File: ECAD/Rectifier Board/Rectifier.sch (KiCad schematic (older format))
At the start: 21 parts

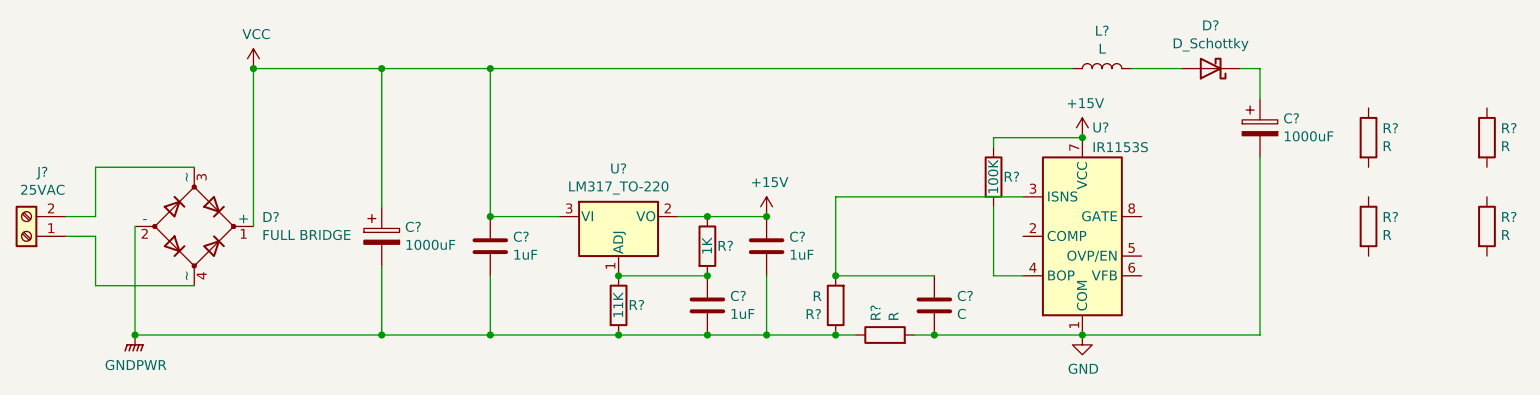
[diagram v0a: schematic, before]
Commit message: Cin
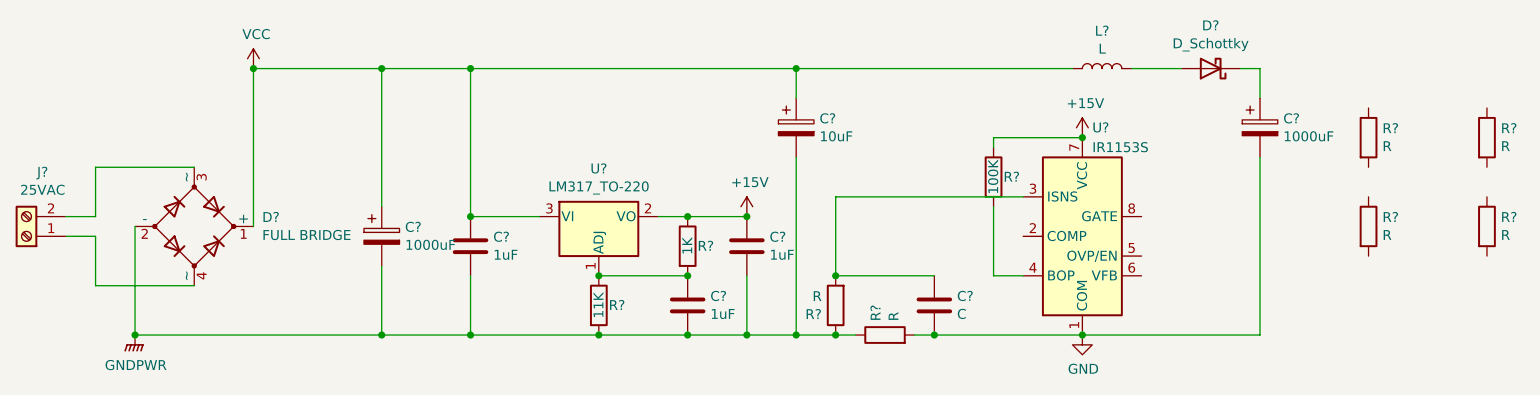
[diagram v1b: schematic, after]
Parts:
- added C?: 10uF, symbol Device:CP
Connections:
- net GNDPWR: now also C?.2
- net VCC: now also C?.1
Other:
- moved on the sheet: C?, R?, U?
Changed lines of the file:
@@
 L Regulator_Linear:LM317_TO-220 U?
 U 1 1 6205D4E8
-P 5150 2900
-F 0 "U?" H 5150 3142 50  0000 C CNN
-F 1 "LM317_TO-220" H 5150 3051 50  0000 C CNN
-F 2 "Package_TO_SOT_THT:TO-220-3_Vertical" H 5150 3150 50  0001 C CIN
-F 3 "http://www.ti.com/lit/ds/symlink/lm317.pdf" H 5150 2900 50  0001 C CNN
-	1    5150 2900
+P 5050 2900
+F 0 "U?" H 5050 3142 50  0000 C CNN
+F 1 "LM317_TO-220" H 5050 3051 50  0000 C CNN
+F 2 "Package_TO_SOT_THT:TO-220-3_Vertical" H 5050 3150 50  0001 C CIN
+F 3 "http://www.ti.com/lit/ds/symlink/lm317.pdf" H 5050 2900 50  0001 C CNN
+	1    5050 2900
 	1    0    0    -1
 $EndComp
@@
 L Device:R R?
 U 1 1 6205E083
-P 5150 3350
-F 0 "R?" H 5200 3350 50  0000 L CNN
-F 1 "11K" V 5150 3350 50  0000 C CNN
-F 2 "" V 5080 3350 50  0001 C CNN
-F 3 "~" H 5150 3350 50  0001 C CNN
-	1    5150 3350
+P 5050 3350
+F 0 "R?" H 5100 3350 50  0000 L CNN
+F 1 "11K" V 5050 3350 50  0000 C CNN
+F 2 "" V 4980 3350 50  0001 C CNN
+F 3 "~" H 5050 3350 50  0001 C CNN
+	1    5050 3350
 	1    0    0    -1
 $EndComp
@@
 L Device:R R?
 U 1 1 6205F378
-P 5600 3050
-F 0 "R?" H 5650 3050 50  0000 L CNN
-F 1 "1K" V 5600 3050 50  0000 C CNN
-F 2 "" V 5530 3050 50  0001 C CNN
-F 3 "~" H 5600 3050 50  0001 C CNN
-	1    5600 3050
-	1    0    0    -1
-$EndComp
-Wire Wire Line
-	5150 3200 5600 3200
-Connection ~ 5150 3200
-Wire Wire Line
-	5600 2900 5450 2900
+P 5500 3050
+F 0 "R?" H 5550 3050 50  0000 L CNN
+F 1 "1K" V 5500 3050 50  0000 C CNN
+F 2 "" V 5430 3050 50  0001 C CNN
+F 3 "~" H 5500 3050 50  0001 C CNN
+	1    5500 3050
+	1    0    0    -1
+$EndComp
+Wire Wire Line
+	5050 3200 5500 3200
+Connection ~ 5050 3200
+Wire Wire Line
+	5500 2900 5350 2900
 $Comp
 L Device:C C?
 U 1 1 6205FE8A
-P 5900 3050
-F 0 "C?" H 6015 3096 50  0000 L CNN
-F 1 "1uF" H 6015 3005 50  0000 L CNN
-F 2 "" H 5938 2900 50  0001 C CNN
-F 3 "~" H 5900 3050 50  0001 C CNN
-	1    5900 3050
+P 5800 3050
+F 0 "C?" H 5915 3096 50  0000 L CNN
+F 1 "1uF" H 5915 3005 50  0000 L CNN
+F 2 "" H 5838 2900 50  0001 C CNN
+F 3 "~" H 5800 3050 50  0001 C CNN
+	1    5800 3050
 	1    0    0    -1
 $EndComp
@@
 L Device:C C?
 U 1 1 620613FC
-P 5600 3350
-F 0 "C?" H 5715 3396 50  0000 L CNN
-F 1 "1uF" H 5715 3305 50  0000 L CNN
-F 2 "" H 5638 3200 50  0001 C CNN
-F 3 "~" H 5600 3350 50  0001 C CNN
-	1    5600 3350
-	1    0    0    -1
-$EndComp
-Connection ~ 5600 3200
-Wire Wire Line
-	5150 3500 5600 3500
-Wire Wire Line
-	5600 3500 5900 3500
-Wire Wire Line
-	5900 3500 5900 3200
-Connection ~ 5600 3500
-Wire Wire Line
-	5900 2900 5600 2900
-Connection ~ 5600 2900
+P 5500 3350
+F 0 "C?" H 5615 3396 50  0000 L CNN
+F 1 "1uF" H 5615 3305 50  0000 L CNN
+F 2 "" H 5538 3200 50  0001 C CNN
+F 3 "~" H 5500 3350 50  0001 C CNN
+	1    5500 3350
+	1    0    0    -1
+$EndComp
+Connection ~ 5500 3200
+Wire Wire Line
+	5800 3500 5800 3200
+Wire Wire Line
+	5800 2900 5500 2900
+Connection ~ 5500 2900
 $Comp
 L Device:C C?
 U 1 1 620625CD
-P 4500 3050
-F 0 "C?" H 4615 3096 50  0000 L CNN
-F 1 "1uF" H 4615 3005 50  0000 L CNN
-F 2 "" H 4538 2900 50  0001 C CNN
-F 3 "~" H 4500 3050 50  0001 C CNN
-	1    4500 3050
-	1    0    0    -1
-$EndComp
-Wire Wire Line
-	4500 3500 4500 3200
-Wire Wire Line
-	4850 2900 4500 2900
-Wire Wire Line
-	4500 3500 5150 3500
-Connection ~ 5150 3500
+P 4400 3050
+F 0 "C?" H 4515 3096 50  0000 L CNN
+F 1 "1uF" H 4515 3005 50  0000 L CNN
+F 2 "" H 4438 2900 50  0001 C CNN
+F 3 "~" H 4400 3050 50  0001 C CNN
+	1    4400 3050
+	1    0    0    -1
+$EndComp
+Wire Wire Line
+	4400 3500 4400 3200
+Wire Wire Line
+	4750 2900 4400 2900
 $Comp
 L Device:CP C?
@@
 	3950 3500 3950 3150
 Wire Wire Line
-	3950 2150 4500 2150
+	3950 2150 4400 2150
 Connection ~ 3950 2150
-Connection ~ 4500 2150
-Wire Wire Line
-	3950 3500 4500 3500
+Wire Wire Line
+	3950 3500 4400 3500
 Connection ~ 3950 3500
-Connection ~ 4500 3500
 $Comp
 L power:+15V #PWR?
 U 1 1 6206D11A
-P 5900 2900
-F 0 "#PWR?" H 5900 2750 50  0001 C CNN
-F 1 "+15V" H 5915 3073 50  0000 C CNN
-F 2 "" H 5900 2900 50  0001 C CNN
-F 3 "" H 5900 2900 50  0001 C CNN
-	1    5900 2900
-	1    0    0    -1
-$EndComp
-Connection ~ 5900 2900
+P 5800 2900
+F 0 "#PWR?" H 5800 2750 50  0001 C CNN
+F 1 "+15V" H 5815 3073 50  0000 C CNN
+F 2 "" H 5800 2900 50  0001 C CNN
+F 3 "" H 5800 2900 50  0001 C CNN
+	1    5800 2900
+	1    0    0    -1
+$EndComp
+Connection ~ 5800 2900
 $Comp
 L power:+15V #PWR?
@@
 Wire Wire Line
 	6250 3500 6350 3500
-Wire Wire Line
-	6250 3500 5900 3500
 Connection ~ 6250 3500
-Connection ~ 5900 3500
 Wire Wire Line
 	6650 3500 6750 3500
 Wire Wire Line
-	4500 2150 4500 2900
-Connection ~ 4500 2900
+	4400 2150 4400 2900
+Connection ~ 4400 2900
 Wire Wire Line
 	3950 2150 3950 2850
@@
 	7050 3200 7200 3200
 Wire Wire Line
-	4500 2150 7450 2150
-Wire Wire Line
 	8400 2300 8400 2150
 Wire Wire Line
@@
 Wire Wire Line
 	8400 3500 7500 3500
+Connection ~ 4400 2150
+Connection ~ 4400 3500
+Connection ~ 5050 3500
+Connection ~ 5500 3500
+Connection ~ 5800 3500
+Wire Wire Line
+	5050 3500 5500 3500
+Wire Wire Line
+	5500 3500 5800 3500
+Wire Wire Line
+	4400 3500 5050 3500
+Wire Wire Line
+	5800 3500 6050 3500
+$Comp
+L Device:CP C?
+U 1 1 621098C4
+P 6050 2450
+F 0 "C?" H 6168 2496 50  0000 L CNN
+F 1 "10uF" H 6168 2405 50  0000 L CNN
+F 2 "" H 6088 2300 50  0001 C CNN
+F 3 "~" H 6050 2450 50  0001 C CNN
+	1    6050 2450
+	1    0    0    -1
+$EndComp
+Wire Wire Line
+	4400 2150 6050 2150
+Wire Wire Line
+	6050 2300 6050 2150
+Connection ~ 6050 2150
+Wire Wire Line
+	6050 2150 7450 2150
+Wire Wire Line
+	6050 2600 6050 3500
+Connection ~ 6050 3500
+Wire Wire Line
+	6050 3500 6250 3500
 $EndSCHEMATC
